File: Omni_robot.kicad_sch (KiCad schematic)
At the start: 85 parts, among them J1 USB_C_Receptacle_USB2.0_16P, J2 Battery_Conn_01x02, J3 M1_Conn_01x06, J4 M1_Conn_01x06, J5 M1_Conn_01x06, SW1 SW_SPDT, SW2 TSC016A04518A, SW4 TSC016A04518A, U1 ESP32-S3-WROOM-1, U2 BQ24074RGT, U3 TPS63060, U4 DRV8833PWP, U5 DRV8833PWP, U7 BMX055, U8 TPD2EUSB30, U9 DRV8833PWP

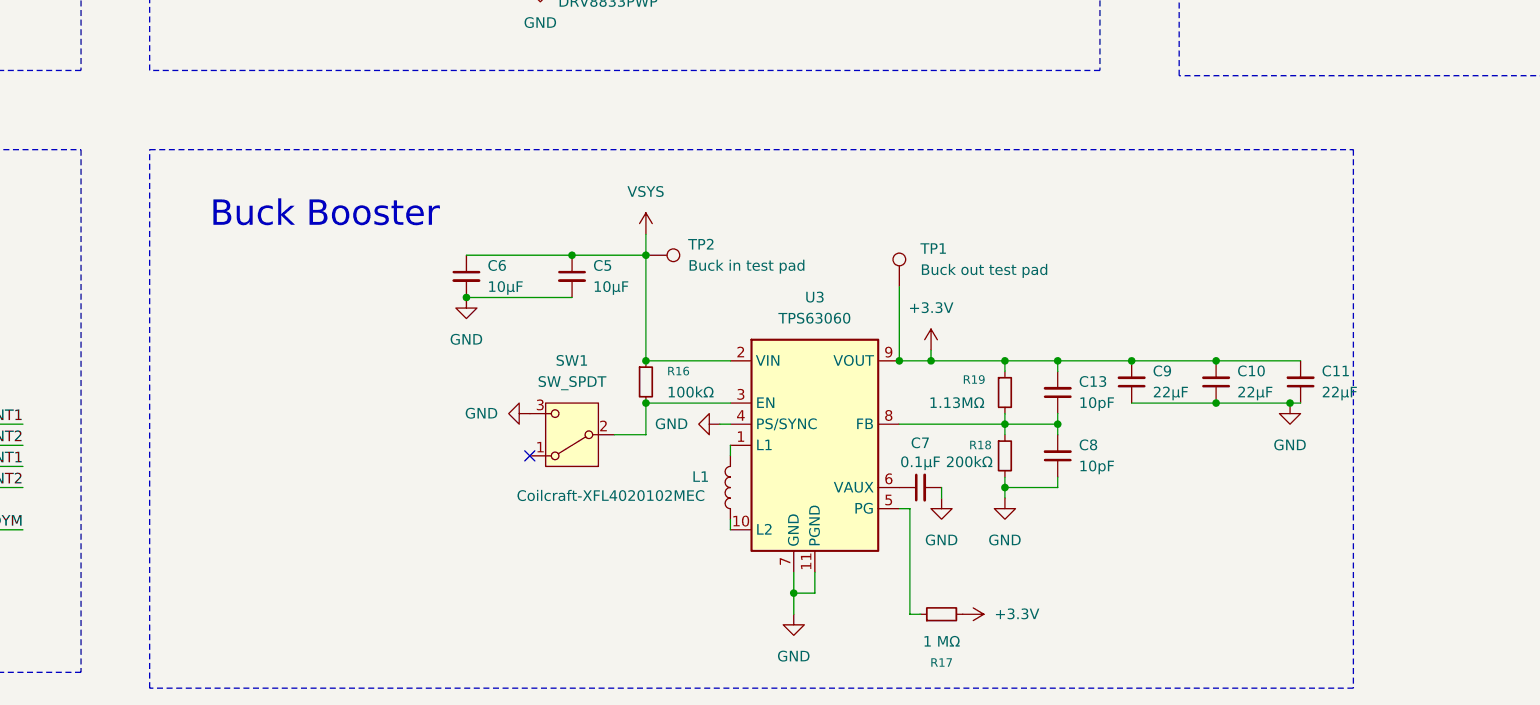
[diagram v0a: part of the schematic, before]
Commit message: Finished basic tracing
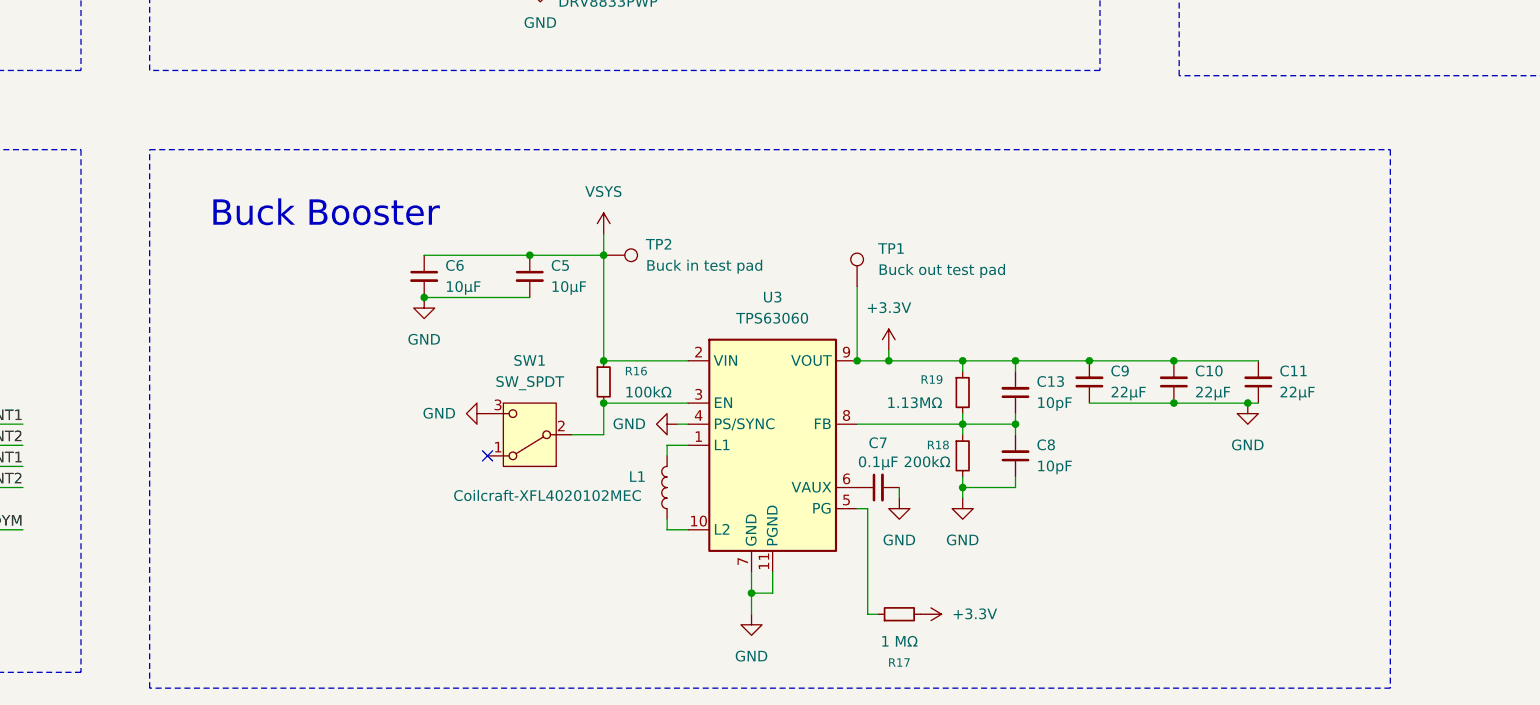
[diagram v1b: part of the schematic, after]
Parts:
- J1: footprint Custom_Connector:USB-C-SMD_TYPE-C16PIN -> Connector_USB:USB_C_Receptacle_Palconn_UTC16-G
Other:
- moved on the sheet: C10, C11, C13, C5, C6, C7, C8, C9, L1, R16, R17, R18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
